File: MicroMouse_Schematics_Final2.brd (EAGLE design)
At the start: 112.7 x 96.3 mm, 64 parts

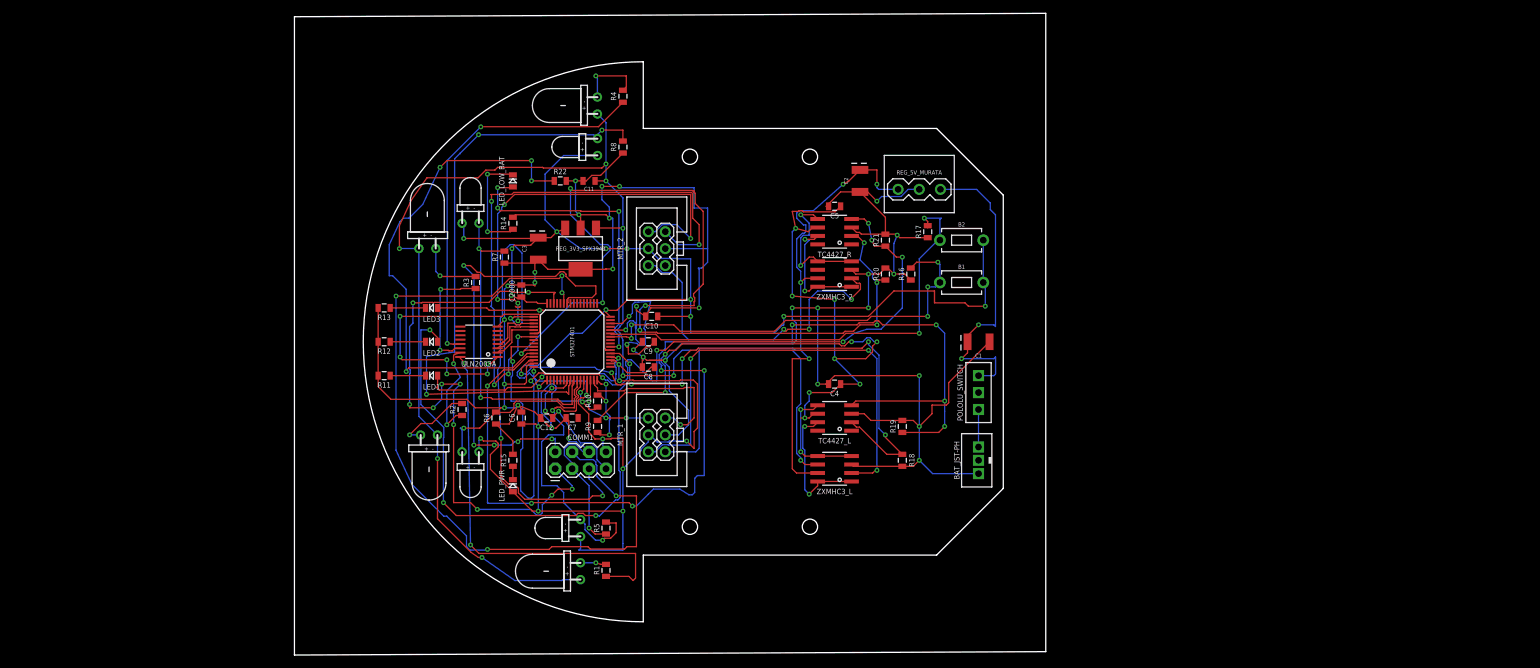
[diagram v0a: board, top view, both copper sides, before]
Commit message: Final Fixed Board
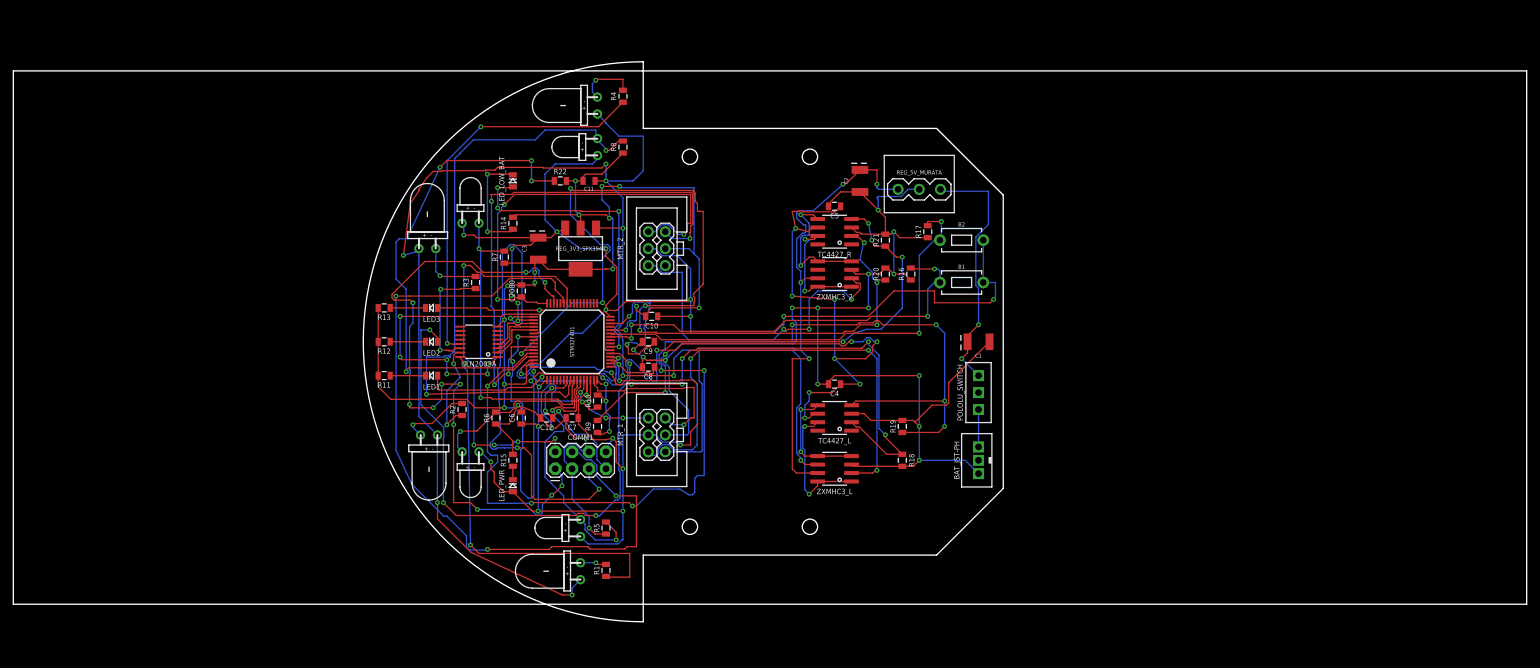
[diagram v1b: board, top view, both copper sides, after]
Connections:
- net +3V3: now also C7.1
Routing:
- net +5V: track 256.8 -> 270.5 mm
- net S$1: track 270.9 -> 260.8 mm
- net TX: track 70.5 -> 61.4 mm
- net SWDIO: track 93.7 -> 102.3 mm, vias 10 -> 11
- net N$3: track 46.3 -> 38.0 mm
- net RENC_B: track 84.8 -> 81.9 mm
- net RE_LF: track 43.6 -> 40.7 mm
- net LMTR+: track 69.8 -> 72.6 mm
- net N$7: track 62.5 -> 60.2 mm
- net +3V3: track 347.8 -> 345.8 mm, vias 23 -> 22
- net LPWM_B: track 170.5 -> 172.4 mm
- net B1: track 70.2 -> 68.4 mm
- net RX: track 119.6 -> 117.9 mm, vias 5 -> 3
- net SWCLK: track 76.4 -> 78.1 mm
- net B0: track 65.1 -> 63.6 mm, vias 5 -> 4
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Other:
- board size 112.7 x 96.3 mm -> 227 x 80 mm

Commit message: Finalized & Ordered PCB with Garber Files
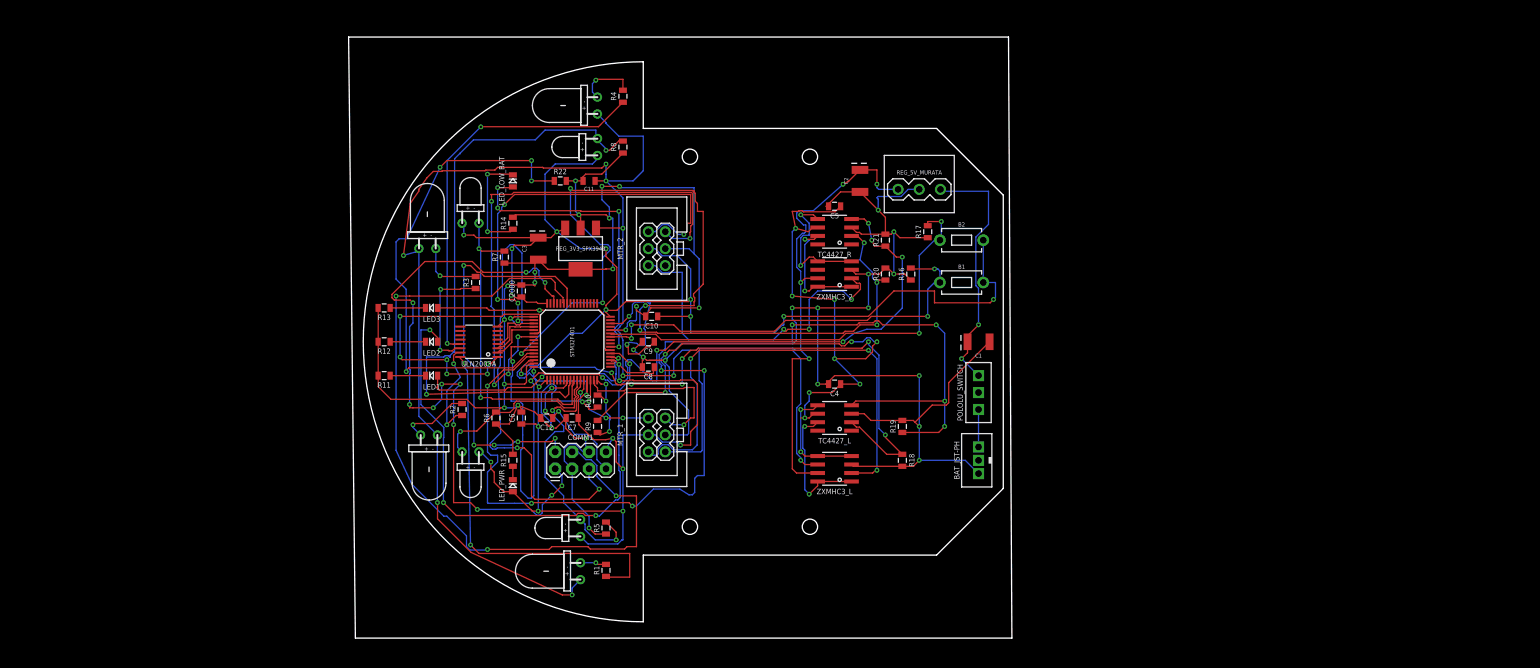
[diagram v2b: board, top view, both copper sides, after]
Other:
- board size 227 x 80 mm -> 99.5 x 90.2 mm
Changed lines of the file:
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@@
 <?xml version="1.0" encoding="utf-8"?>
 <!DOCTYPE eagle SYSTEM "eagle.dtd">
-<eagle version="8.6.0">
+<eagle version="8.7.0">
 <drawing>
 <settings>
@@
 <board>
 <plain>
-<wire x1="0" y1="0" x2="227" y2="0" width="0" layer="20"/>
-<wire x1="227" y1="0" x2="227" y2="80" width="0" layer="20"/>
-<wire x1="227" y1="80" x2="0" y2="80" width="0" layer="20"/>
-<wire x1="0" y1="80" x2="0" y2="0" width="0" layer="20"/>
+<wire x1="51.308" y1="-5.08" x2="149.784" y2="-5.08" width="0" layer="20"/>
+<wire x1="149.784" y1="-5.08" x2="149.276" y2="85.08" width="0" layer="20"/>
+<wire x1="149.276" y1="85.08" x2="50.292" y2="85.08" width="0" layer="20"/>
+<wire x1="50.292" y1="85.08" x2="51.308" y2="-5.08" width="0" layer="20"/>
 </plain>
 <attributes>
